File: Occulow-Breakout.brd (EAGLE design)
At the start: 49.5 x 50.8 mm, 18 parts

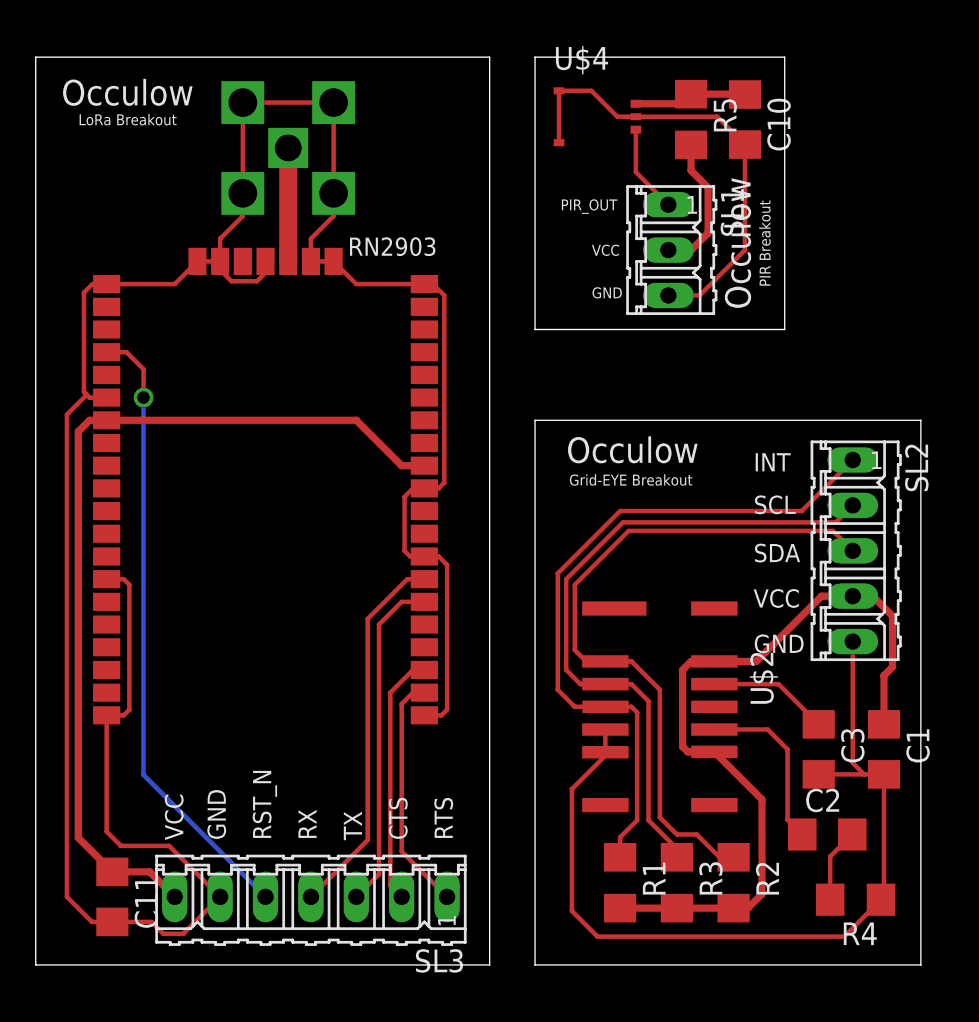
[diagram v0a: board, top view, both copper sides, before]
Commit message: Rename caps, bom
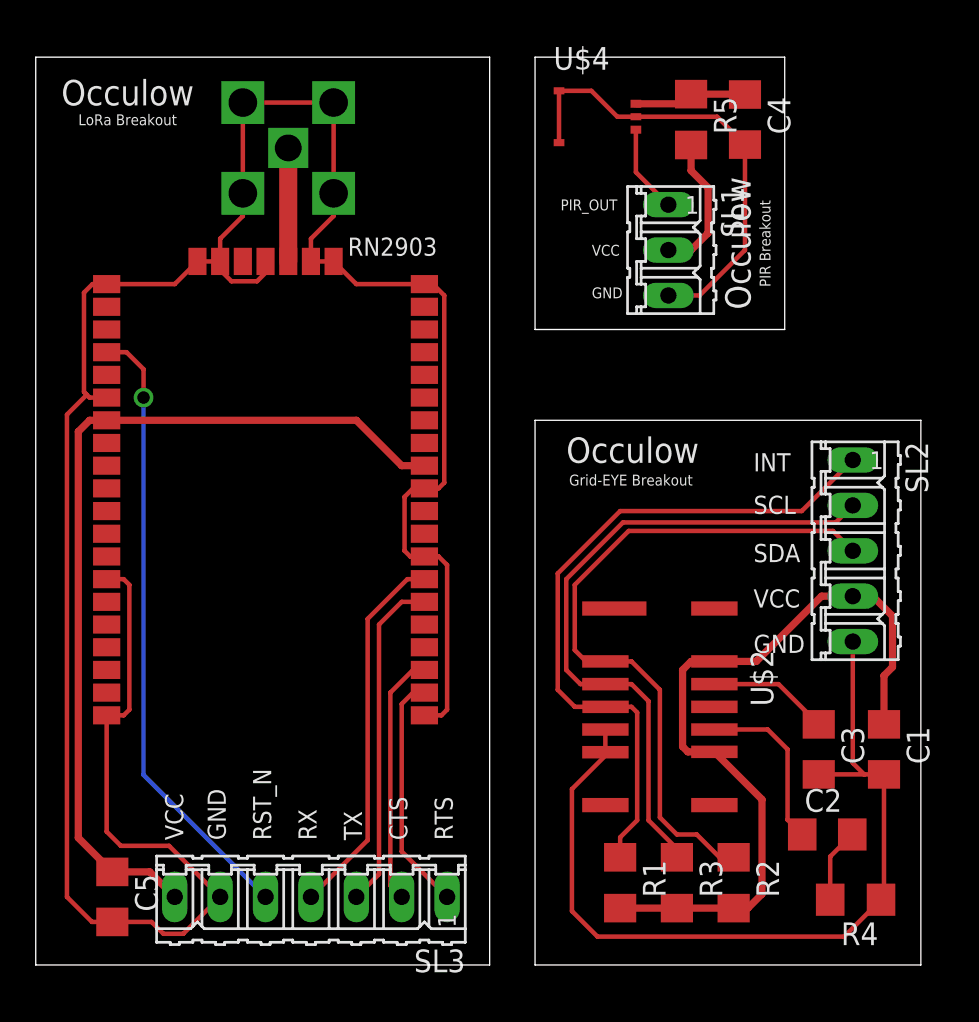
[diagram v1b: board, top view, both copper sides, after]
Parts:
- renumbered C10 to C4, C11 to C5
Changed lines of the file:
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@@
 <?xml version="1.0" encoding="utf-8"?>
 <!DOCTYPE eagle SYSTEM "eagle.dtd">
-<eagle version="8.0.0">
+<eagle version="8.0.2">
 <drawing>
 <settings>
@@
 <element name="U$3" library="SMA-JACK" package="SMA-JACK" value="SMA-JACKFEMALE" x="14.12875" y="45.72"/>
 <element name="U$4" library="PIR" package="IRS-B210ST01" value="IRS-B210ST01" x="31.4325" y="47.46625"/>
-<element name="C10" library="rcl" package="C1206" value="100uF" x="39.6875" y="47.3075" rot="R270"/>
+<element name="C4" library="rcl" package="C1206" value="100uF" x="39.6875" y="47.3075" rot="R270"/>
 <element name="R5" library="resistor" package="R1206" value="619k" x="36.67125" y="47.3075" rot="R270"/>
-<element name="C11" library="rcl" package="C1206" value="10uF" x="4.28625" y="3.81" rot="R270"/>
+<element name="C5" library="rcl" package="C1206" value="10uF" x="4.28625" y="3.81" rot="R270"/>
 <element name="SL1" library="con-amp-quick" package="03P" value="" x="35.40125" y="40.005" rot="R270">
 <attribute name="MF" value="" x="35.40125" y="40.005" size="1.778" layer="27" rot="R270" display="off"/>
+<attribute name="MPN" value="" x="35.40125" y="40.005" size="1.778" layer="27" rot="R270" display="off"/>
 <attribute name="OC_FARNELL" value="unknown" x="35.40125" y="40.005" size="1.778" layer="27" rot="R270" display="off"/>
 <attribute name="OC_NEWARK" value="unknown" x="35.40125" y="40.005" size="1.778" layer="27" rot="R270" display="off"/>
-<attribute name="MPN" value="" x="35.40125" y="40.005" size="1.778" layer="27" rot="R270" display="off"/>
 </element>
 <element name="SL2" library="con-amp-quick" package="05P" value="" x="45.72" y="23.1775" rot="R270">
 <attribute name="MF" value="" x="45.72" y="23.1775" size="1.778" layer="27" rot="R270" display="off"/>
+<attribute name="MPN" value="" x="45.72" y="23.1775" size="1.778" layer="27" rot="R270" display="off"/>
 <attribute name="OC_FARNELL" value="unknown" x="45.72" y="23.1775" size="1.778" layer="27" rot="R270" display="off"/>
 <attribute name="OC_NEWARK" value="unknown" x="45.72" y="23.1775" size="1.778" layer="27" rot="R270" display="off"/>
-<attribute name="MPN" value="" x="45.72" y="23.1775" size="1.778" layer="27" rot="R270" display="off"/>
 </element>
 <element name="SL3" library="con-amp-quick" package="07P" value="" x="15.39875" y="3.81" rot="R180">
 <attribute name="MF" value="" x="15.39875" y="3.81" size="1.778" layer="27" rot="R180" display="off"/>
+<attribute name="MPN" value="" x="15.39875" y="3.81" size="1.778" layer="27" rot="R180" display="off"/>
 <attribute name="OC_FARNELL" value="unknown" x="15.39875" y="3.81" size="1.778" layer="27" rot="R180" display="off"/>
 <attribute name="OC_NEWARK" value="unknown" x="15.39875" y="3.81" size="1.778" layer="27" rot="R180" display="off"/>
-<attribute name="MPN" value="" x="15.39875" y="3.81" size="1.778" layer="27" rot="R180" display="off"/>
 </element>
 </elements>
@@
 <signal name="N$5">
 <contactref element="U$4" pad="3"/>
-<contactref element="C10" pad="1"/>
+<contactref element="C4" pad="1"/>
 <contactref element="R5" pad="1"/>
 <wire x1="33.5825" y1="48.19125" x2="36.133" y2="48.19125" width="0.4064" layer="1"/>
@@
 <contactref element="U$1" pad="12"/>
 <contactref element="U$1" pad="34"/>
-<contactref element="C11" pad="1"/>
+<contactref element="C5" pad="1"/>
 <contactref element="SL3" pad="7"/>
 <wire x1="21.74875" y1="27.94" x2="20.47875" y2="27.94" width="0.4064" layer="1"/>
@@
 <contactref element="U$4" pad="5"/>
 <contactref element="U$4" pad="2"/>
-<contactref element="C10" pad="2"/>
+<contactref element="C4" pad="2"/>
 <contactref element="SL1" pad="3"/>
 <wire x1="29.2825" y1="46.01625" x2="29.2825" y2="48.91625" width="0.254" layer="1"/>
@@
 <contactref element="U$1" pad="41"/>
 <contactref element="U$1" pad="47"/>
-<contactref element="C11" pad="2"/>
+<contactref element="C5" pad="2"/>
 <contactref element="U$1" pad="20"/>
 <contactref element="U$1" pad="11"/>
